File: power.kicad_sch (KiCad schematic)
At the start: 41 parts, among them U1 74HC86, U10 74AHC30, U11 74AHC30, U12 74AHC30, U13 74AHC30, U15 74LV32, U16 74HC109, U17 74LV32, U18 74LV04, U19 74LV08, U2 74HC00, U21 74AHC30, U22 74AHC30, U23 74AHC30, U24 74AHC30, U25 74HC109, U3 74LV27, U30 74LV08, U31 74LV08, U4 74HC00

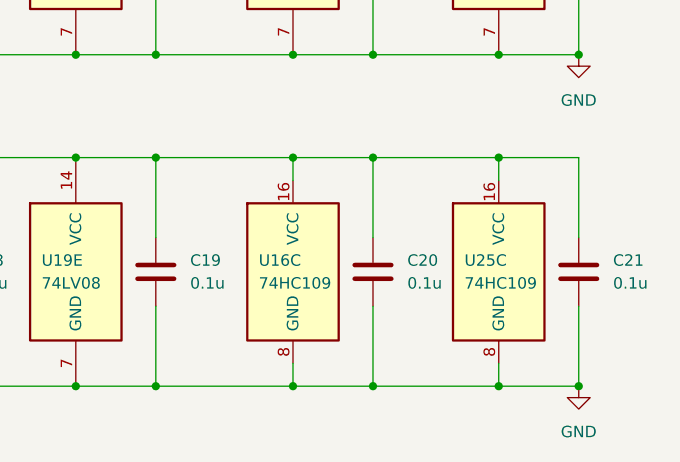
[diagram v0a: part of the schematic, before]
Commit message: Memory routing *screams*
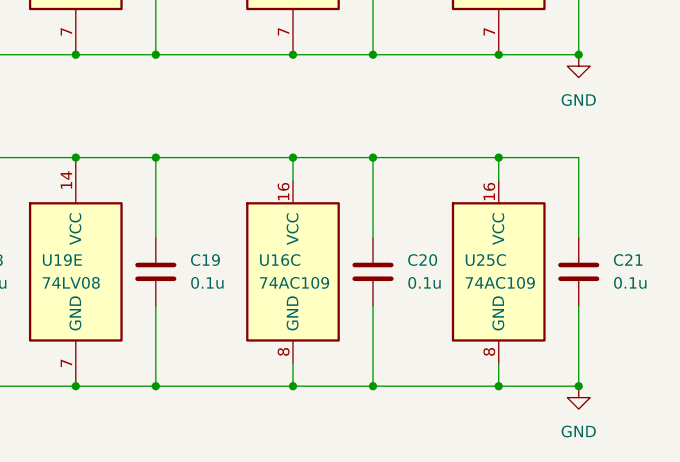
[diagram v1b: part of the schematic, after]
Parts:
- U16, U25: value 74HC109 -> 74AC109
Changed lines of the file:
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@@
       (effects (font (size 1.27 1.27)) (justify left))
     )
-    (property "Value" "74HC109" (at 166.37 118.11 0)
+    (property "Value" "74AC109" (at 166.37 118.11 0)
       (effects (font (size 1.27 1.27)) (justify left))
     )
@@
       (effects (font (size 1.27 1.27)) (justify left))
     )
-    (property "Value" "74HC109" (at 189.23 118.11 0)
-      (effects (font (size 1.27 1.27)) (justify left))
-    )
+    (property "Value" "74AC109" (at 189.23 118.11 0)
+      (effects (font (size 1.27 1.27)) (justify left))
+    )
